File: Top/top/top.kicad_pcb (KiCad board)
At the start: 2 copper layers, 45 x 45 mm, 11 parts, among them J1 Conn_02x08_Odd_Even, J2 Conn_01x10_Female, J3 Header, J4 JST Connector

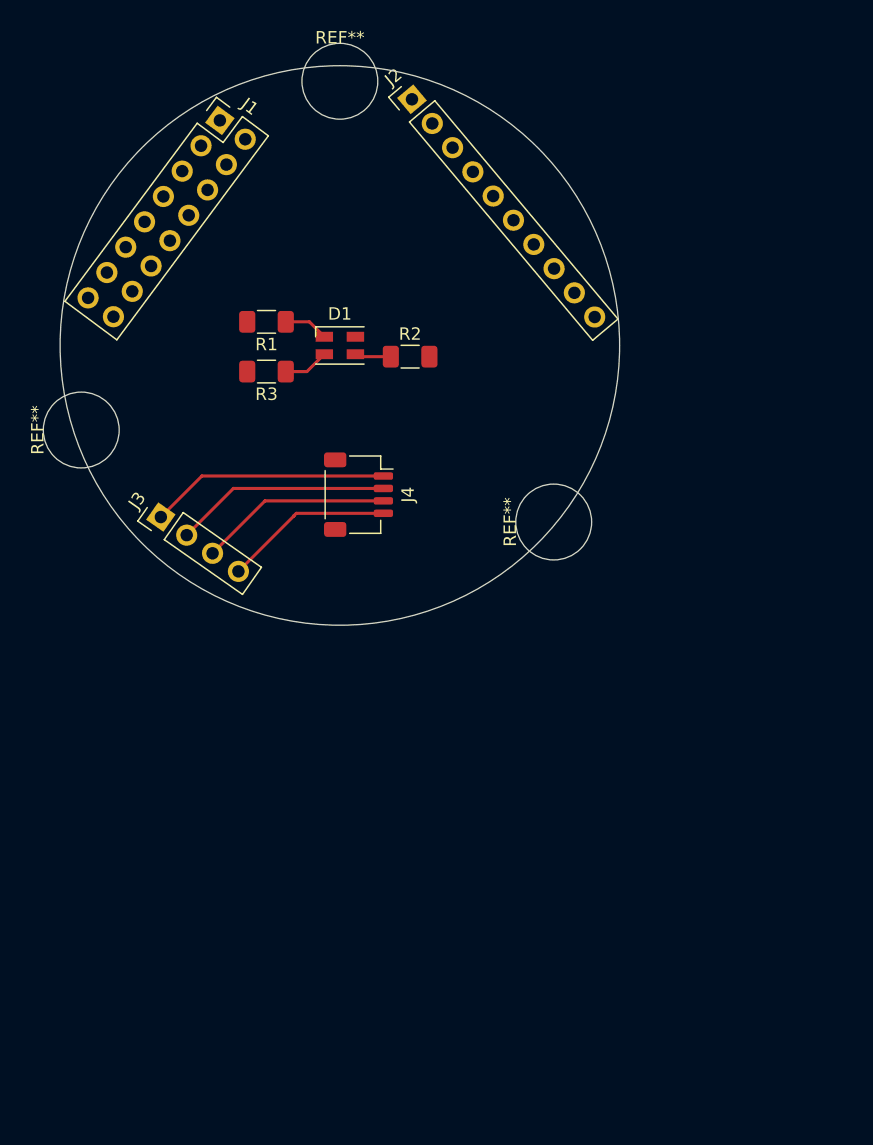
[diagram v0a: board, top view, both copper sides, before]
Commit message: Version 0.1.7 - Various changes, see changelog
Signed-off-by: ray33ee <30669752+ray33ee@users.noreply.github.com>
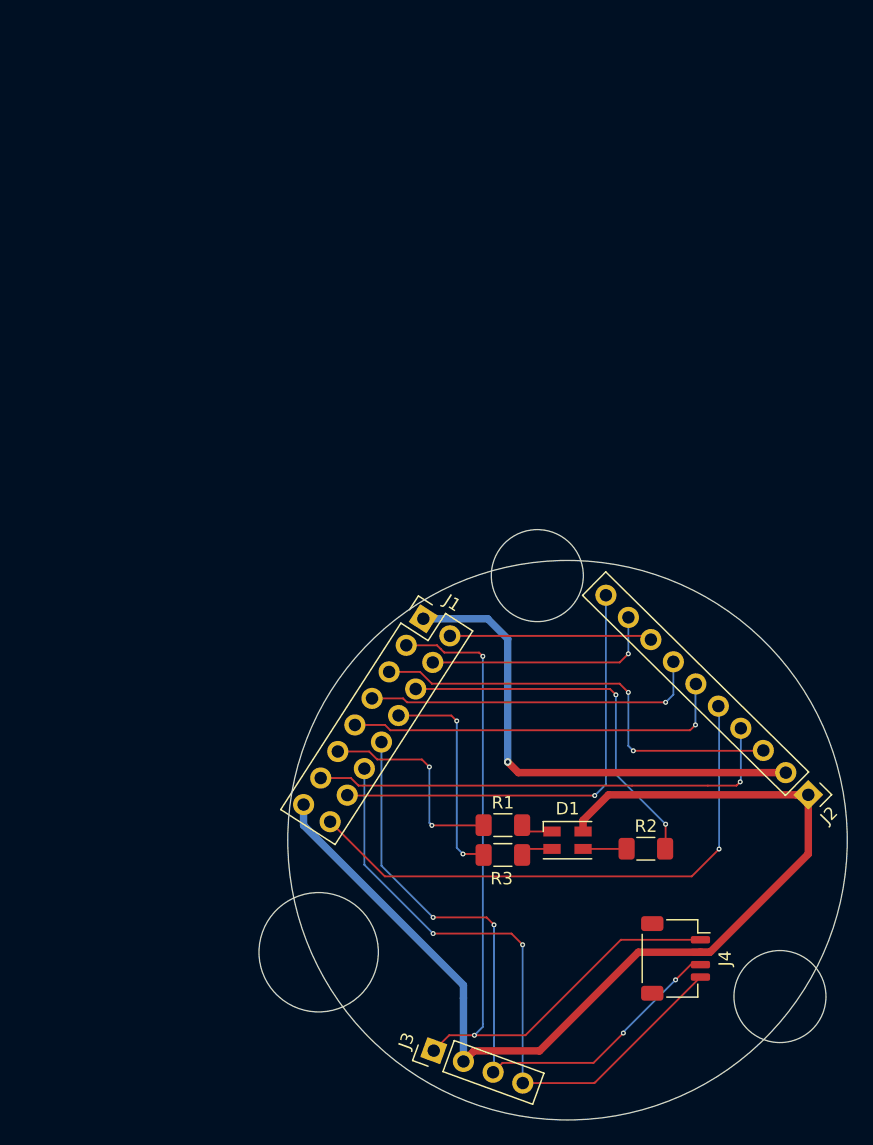
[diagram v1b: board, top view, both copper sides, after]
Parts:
- removed REF** (x3): MountingHole_2.5mm, MountingHole:MountingHole_2.5mm
- added MH1: GenericMountingHole, MountingHole:GenericMountingHole, F.Cu at (155.8, 111.8)
- added MH2: GenericMountingHole, MountingHole:GenericMountingHole, F.Cu at (138.2, 142.1)
- added MH3: GenericMountingHole, MountingHole:GenericMountingHole, F.Cu at (175.3, 145.7)
- moved J2 64.4 mm to (177.6, 129.4), turned to 225.4 degrees
- moved J3 48.2 mm to (147.5, 150.0), turned to 70 degrees
- moved J4 45.2 mm to (166.9, 142.6)
- moved R1 44.7 mm to (153.0, 131.9)
- moved R2 43.9 mm to (164.5, 133.8)
- moved D1 43.8 mm to (158.2, 133.1)
- moved J1 43.3 mm to (146.6, 115.3), turned to 327.2 degrees
- moved R3 43.3 mm to (153.0, 134.3)
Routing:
- net GND: track 17.4 -> 86.2 mm
- net /Enabled_Controlled: track 0.00 -> 45.5 mm, vias 0 -> 1
- net +3V3: track 19.3 -> 62.4 mm, vias 0 -> 2
- net +5V: track 0.00 -> 40.1 mm, vias 0 -> 1
- net /SDA: track 13.6 -> 52.1 mm, vias 0 -> 2
- net /PushButton: track 0.00 -> 38.4 mm, vias 0 -> 1
- net /SCL: track 15.5 -> 53.2 mm, vias 0 -> 4
- net /Coil_A1: track 0.00 -> 36.4 mm, vias 0 -> 1
- net /Coil_B2: track 0.00 -> 35.3 mm, vias 0 -> 2
- net /Diff_P1: track 0.00 -> 31.1 mm, vias 0 -> 1
- net /LED_Green: track 0.00 -> 30.4 mm, vias 0 -> 2
- net /Diff_P2: track 0.00 -> 27.3 mm, vias 0 -> 1
- net /Coil_A2: track 0.00 -> 18.9 mm, vias 0 -> 1
- net /LED_Blue: track 0.00 -> 17.5 mm, vias 0 -> 2
- net /LED_Red: track 0.00 -> 16.8 mm, vias 0 -> 2
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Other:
- net class Default: clearance 0.2 -> 0.127; trace_width 0.25 -> 0.15; via_dia 0.8 -> 0.4; via_drill 0.4 -> 0.2
- net class High Current added: clearance 0.15, trace_width 0.6, via_dia 0.6, via_drill 0.3
- rule trace_clearance: 0.2 -> 0.127
- rule trace_min: 0.2 -> 0.127
- rule via_min_drill: 0.3 -> 0.2
